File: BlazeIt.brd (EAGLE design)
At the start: 100 x 80 mm, 38 parts, among them IC1 L293D, IC2 L293D, Q1 200mA/40V, Q2 200mA/40V, Q3 200mA/40V, Q4 200mA/40V, U3 LM317

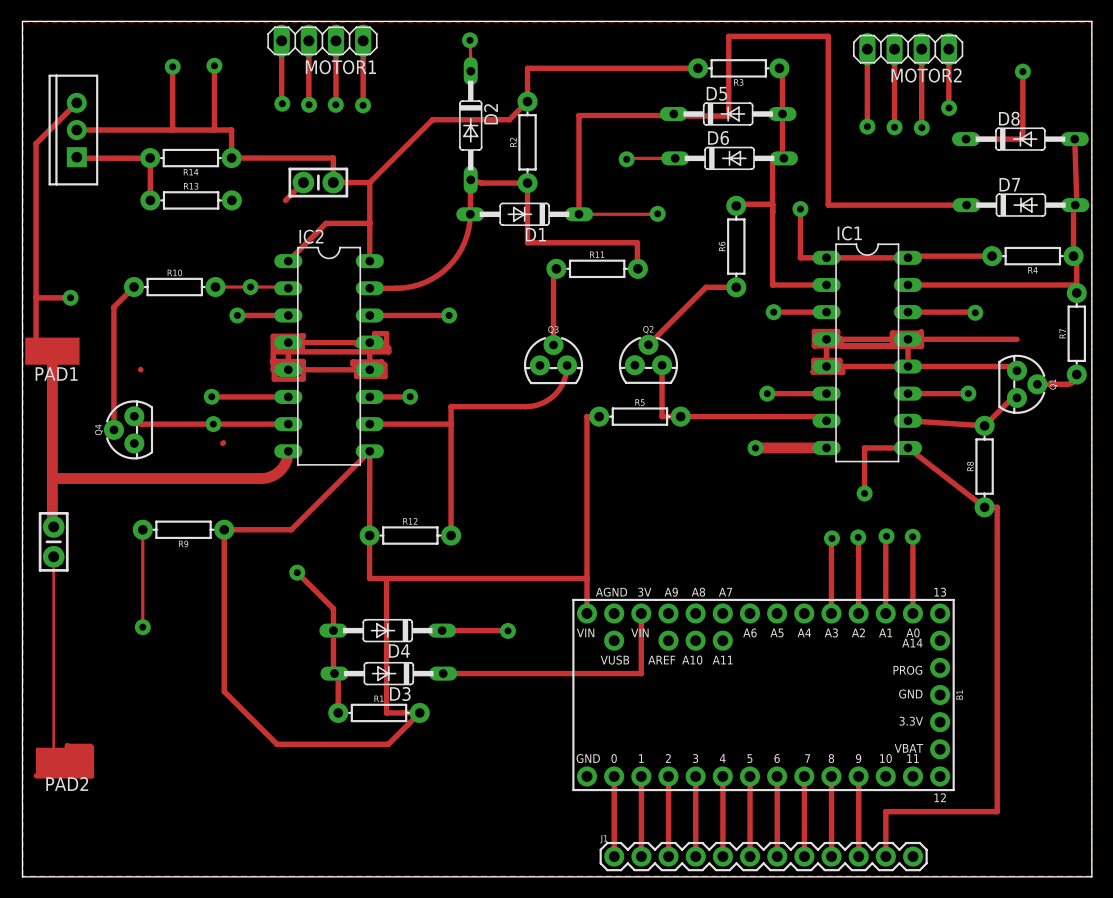
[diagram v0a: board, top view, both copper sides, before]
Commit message: Final final design
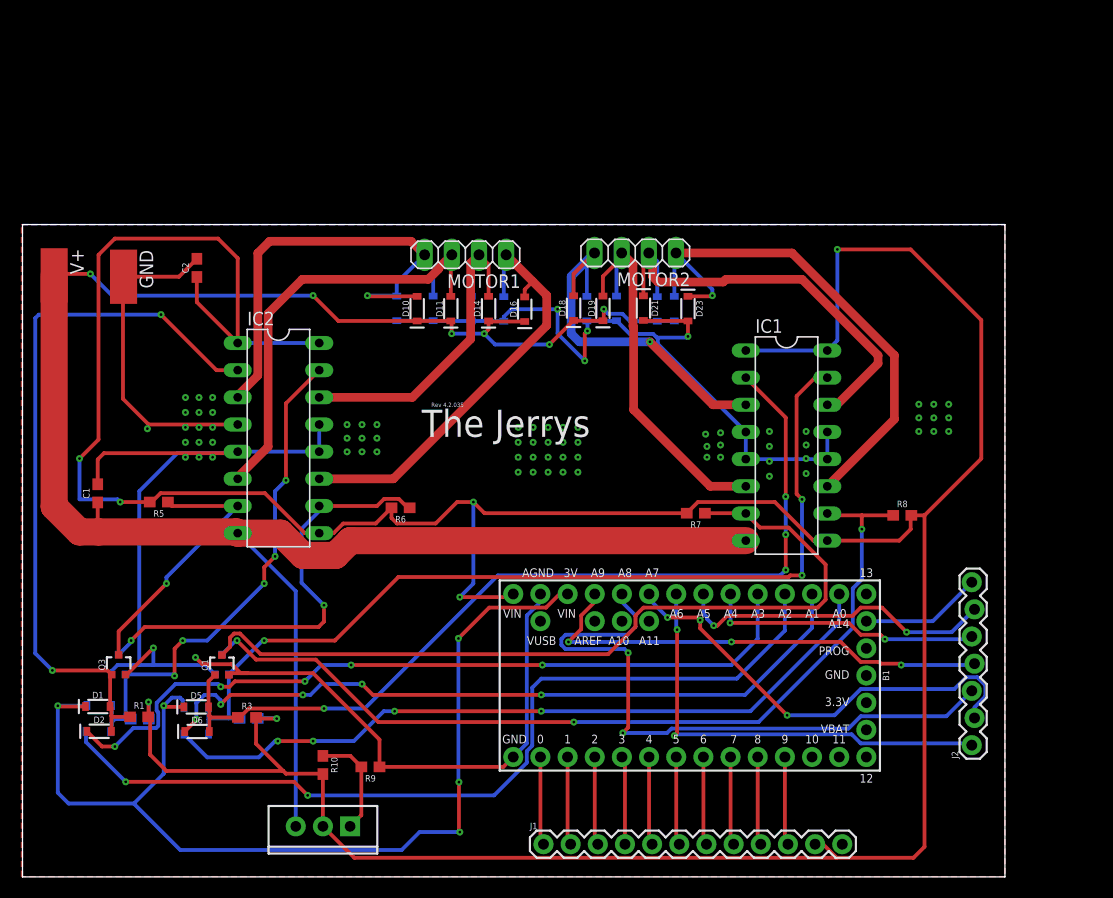
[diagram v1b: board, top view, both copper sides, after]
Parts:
- removed PAD1: 14V, wirepad:SMD2,54-5,08
- removed PAD2: GND PAD, wirepad:SMD2,54-5,08
- removed R11, R13: 1k, SparkFun-Resistors:AXIAL-0.3
- removed R12: 10k, SparkFun-Resistors:AXIAL-0.3
- removed R14: 330, SparkFun-Resistors:AXIAL-0.3
- added D10, D11, D12, D13, D14, D15, D16, D17, D18, D19, D20, D21, D22, D23, D24, D9: (no value), SparkFun-DiscreteSemi:SOD-323
- added GND: GND PAD, wirepad:SMD2,54-5,08
- added J2: (no value), SparkFun-Connectors:1X07_LOCK
- added V+: 14V, wirepad:SMD2,54-5,08
- C1, C2: device SparkFun-Capacitors:CAP-PTH-SMALL-KIT -> SparkFun-Capacitors:0603
- D1, D2, D3, D4, D5, D6, D7, D8: value 1N4148DO35-10 -> (none); device diode:DO35-10 -> SparkFun-DiscreteSemi:SOD-323
- Q1, Q2, Q3, Q4: value 200mA/40V -> (none); device SparkFun-DiscreteSemi:TO-92 -> SparkFun-DiscreteSemi:SOT323
- R1, R2, R3, R4, R5, R8: device SparkFun-Resistors:AXIAL-0.3 -> SparkFun-Resistors:0603
- R10: value 1k -> 330; device SparkFun-Resistors:AXIAL-0.3 -> SparkFun-Resistors:0603
- R6, R7: value 1k -> 10k; device SparkFun-Resistors:AXIAL-0.3 -> SparkFun-Resistors:0603
- R9: value 10k -> 1k; device SparkFun-Resistors:AXIAL-0.3 -> SparkFun-Resistors:0603
- moved D8 95.1 mm to (16.2, 13.3), flipped to the bottom, turned to 180 degrees
- moved D7 90.3 mm to (16.3, 15.8), flipped to the bottom, turned to 180 degrees
- moved R4 85.1 mm to (21.1, 14.8), flipped to the bottom
- moved Q1 78.9 mm to (18.6, 19.8), turned to 0 degrees
- moved R3 76.2 mm to (21.0, 14.9), turned to 0 degrees
- moved D5 74.5 mm to (16.2, 15.9)
- moved D6 73.2 mm to (16.3, 13.6)
- moved U3 69.1 mm to (28.1, 4.73), turned to 180 degrees
- moved D2 66.5 mm to (7.17, 13.6), turned to 0 degrees
- moved R2 65.0 mm to (11.0, 14.8), flipped to the bottom, turned to 180 degrees
- moved D1 60.9 mm to (7.04, 15.9), turned to 0 degrees
- moved Q3 49.4 mm to (8.99, 19.8)
- moved Q2 48.7 mm to (18.6, 19.9), flipped to the bottom
- moved R10 46.8 mm to (28.1, 10.5), turned to 270 degrees
- moved R5 45.7 mm to (12.8, 35.1), turned to 180 degrees
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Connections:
- removed net N$10: Q2.2, R6.P$1
- removed net N$15: IC1.7, Q2.3, R5.P$2
- removed net N$16: IC1.14, MOTOR2.2
- removed net N$17: IC1.10, Q1.3, R8.P$2
- removed net N$2: IC1.3, MOTOR2.3
- removed net N$20: Q1.2, R7.P$1
- removed net N$22: Q4.2, R10.P$1
- removed net N$23: IC2.7, Q4.3, R9.P$2
- removed net N$26: IC2.6, MOTOR1.4
- removed net N$27: IC2.14, MOTOR1.2
- removed net N$28: IC2.10, Q3.3, R12.P$2
- removed net N$3: IC2.11, MOTOR1.1
- removed net N$30: Q3.2, R11.P$1
- removed net N$4: IC1.6, MOTOR2.4
- removed net N$5: IC1.11, MOTOR2.1
- new net EXPANSION1: B1.20, J2.1
- new net EXPANSION2: B1.21, J2.2
- new net EXPANSION3: B1.22, J2.3
- new net EXPANSION4: B1.23, J2.4
- new net EXPANSION5: B1.18, J2.5
- new net EXPANSION6: B1.19, J2.6
- new net EXPANSION7: B1.A14/DAC, J2.7
- new net INPUT1: IC2.7, Q3.3, R5.1
- new net INPUT2: IC2.10, Q4.3, R6.1
- new net INPUT3: IC1.7, Q1.3, R7.1
- new net INPUT4: IC1.10, Q2.3, R8.1
- new net PIN1: D10.A, D9.C, IC2.3, MOTOR1.4
- new net PIN2: D11.A, D12.C, IC2.6, MOTOR1.3
- new net PIN3: D13.C, D14.A, IC2.14, MOTOR1.2
- new net PIN4: D15.C, D16.A, IC2.11, MOTOR1.1
- new net PIN5: D17.C, D18.A, IC1.3, MOTOR2.4
- new net PIN6: D19.A, D20.C, IC1.6, MOTOR2.3
- new net PIN7: D21.C, D22.A, IC1.14, MOTOR2.2
- new net PIN8: D23.C, D24.A, IC1.11, MOTOR2.1
- net 12V: now also D10.C, D11.C, D14.C, D16.C, D18.C, D19.C, D22.C, D24.C, V+.1; no longer PAD1.1
- net 3.3V: no longer B1.3.3V
- net 5V: now also R1.2, R10.2, R2.2, R3.2, R4.2, R5.2, R6.2, R7.2, R8.2; no longer R1.P$2, R12.P$1, R14.P$1, R2.P$2, R3.P$2, R4.P$2, R5.P$1, R8.P$1, R9.P$1
- net CONTROL1: now also D2.C; no longer D4.C
- net CONTROL2: now also D4.C; no longer D2.C
- net GND: now also D12.A, D13.A, D15.A, D17.A, D20.A, D21.A, D23.A, D9.A, GND.1, Q1.2, Q2.2, Q3.2, Q4.2, R9.1; no longer PAD2.1, Q1.1, Q2.1, Q3.1, Q4.1, R13.P$2
- net MOTOR1: now also D1.A, D2.A, Q3.1, R1.1; no longer D3.A, D4.A, R1.P$1, R10.P$2
- net MOTOR2: now also D3.A, D4.A, Q4.1, R2.1; no longer D1.A, D2.A, R11.P$2, R2.P$1
- net MOTOR3: now also Q1.1, R3.1; no longer R3.P$1, R6.P$2
- net MOTOR4: now also Q2.1, R4.1; no longer R4.P$1, R7.P$2
- net N$1: now also B1.3.3V; no longer IC2.3, MOTOR1.3
- net N$6: now also R10.1, R9.2; no longer R13.P$1, R14.P$2
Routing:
- net 12V: track 74.4 -> 189.9 mm, vias 2 -> 6
- net INPUT4: track 0.00 -> 83.5 mm, vias 0 -> 3
- net INPUT3: track 0.00 -> 77.9 mm
- net CONTROL2: track 10.8 -> 82.0 mm
- net CONTROL1: track 13.2 -> 73.5 mm, vias 2 -> 5
- net EXPANSION3: track 0.00 -> 60.1 mm, vias 0 -> 2
- net CONTROL3: track 11.8 -> 68.6 mm, vias 2 -> 5
- net MOTOR4: track 31.2 -> 87.5 mm, vias 0 -> 3
- net MOTOR3: track 31.1 -> 84.8 mm, vias 0 -> 4
- net CONTROL4: track 18.8 -> 70.1 mm, vias 2 -> 4
- net PIN8: track 0.00 -> 51.1 mm, vias 0 -> 1
- net MOTOR1: track 21.8 -> 67.7 mm
- net 5V: track 302.5 -> 347.7 mm, vias 4 -> 7
- net PIN2: track 0.00 -> 44.5 mm
- net EXPANSION4: track 0.00 -> 44.4 mm, vias 0 -> 3
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- added copper zone on layer 16, net GND
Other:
- board size 100 x 80 mm -> 91.9 x 61 mm
- board text added: "Rev 4.2.035"
- board text added: "The Jerrys"
